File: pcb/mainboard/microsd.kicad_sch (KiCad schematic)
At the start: 11 parts, among them U700 W25Q128JVP

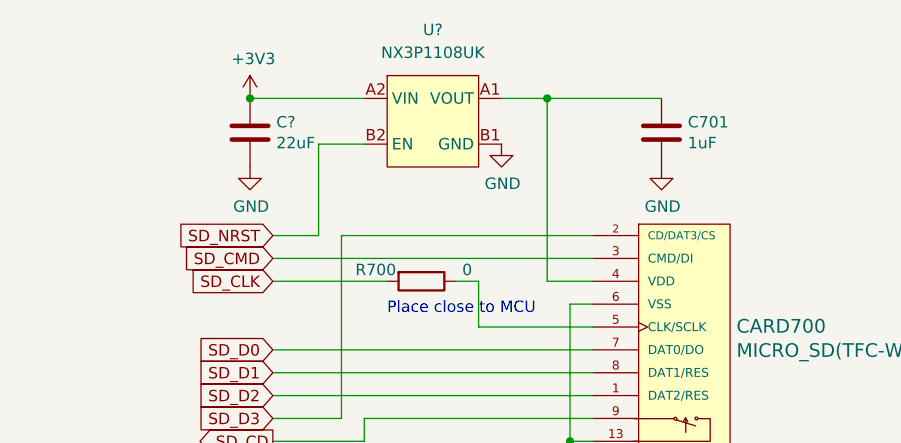
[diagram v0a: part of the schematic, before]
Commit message: Working on mainboard schematics
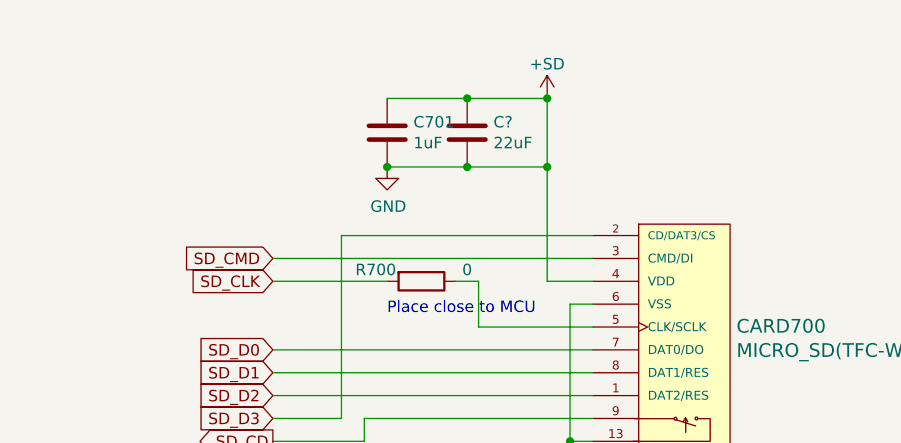
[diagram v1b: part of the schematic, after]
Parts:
- removed U?: NX3P1108UK, footprint:CSP-4_2x2_1.0x1.0mm, symbol symbols:NX3P1108UK
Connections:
- net +3V3 is gone; now on net +SD: C?.1
- net GND is gone; now on net +SD: C701.2, C703.1, C?.1, C?.2, CARD700.10, CARD700.11, CARD700.12, CARD700.13, CARD700.6 (VSS), U700.4 (GND), U700.9 (EP)
- net +SD: now reaches C701.1, CARD700.4 (VDD)
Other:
- moved on the sheet: C701, C?
